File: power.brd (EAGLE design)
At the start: 120 x 120 mm, 34 parts, among them CN1 21700, CN2 21700, CN5 15PIN 0.5MM, Q1 IRLML6244, Q2 IRLML6244, U1 MAX17320G20+

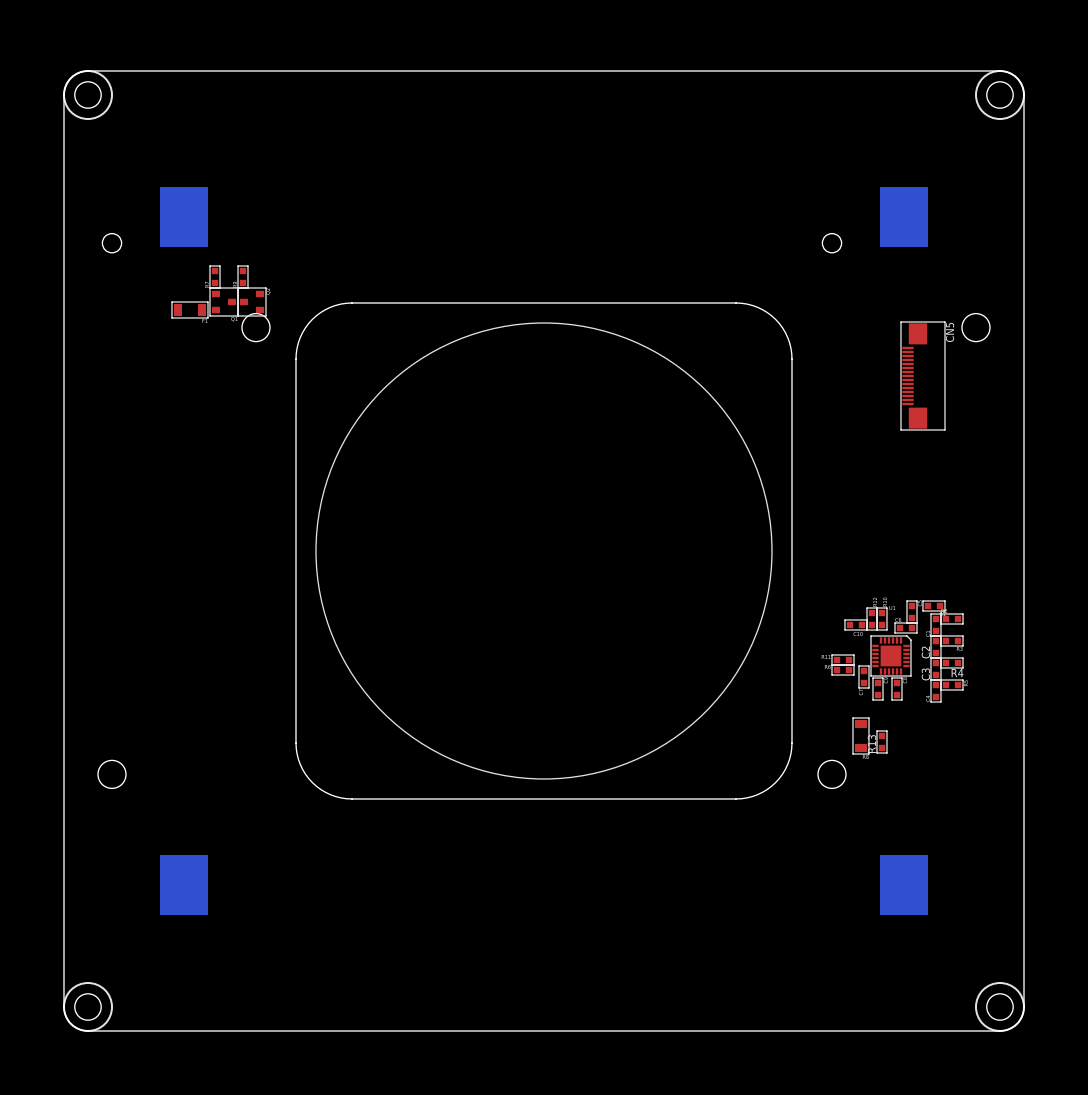
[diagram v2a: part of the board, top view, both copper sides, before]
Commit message: Progress
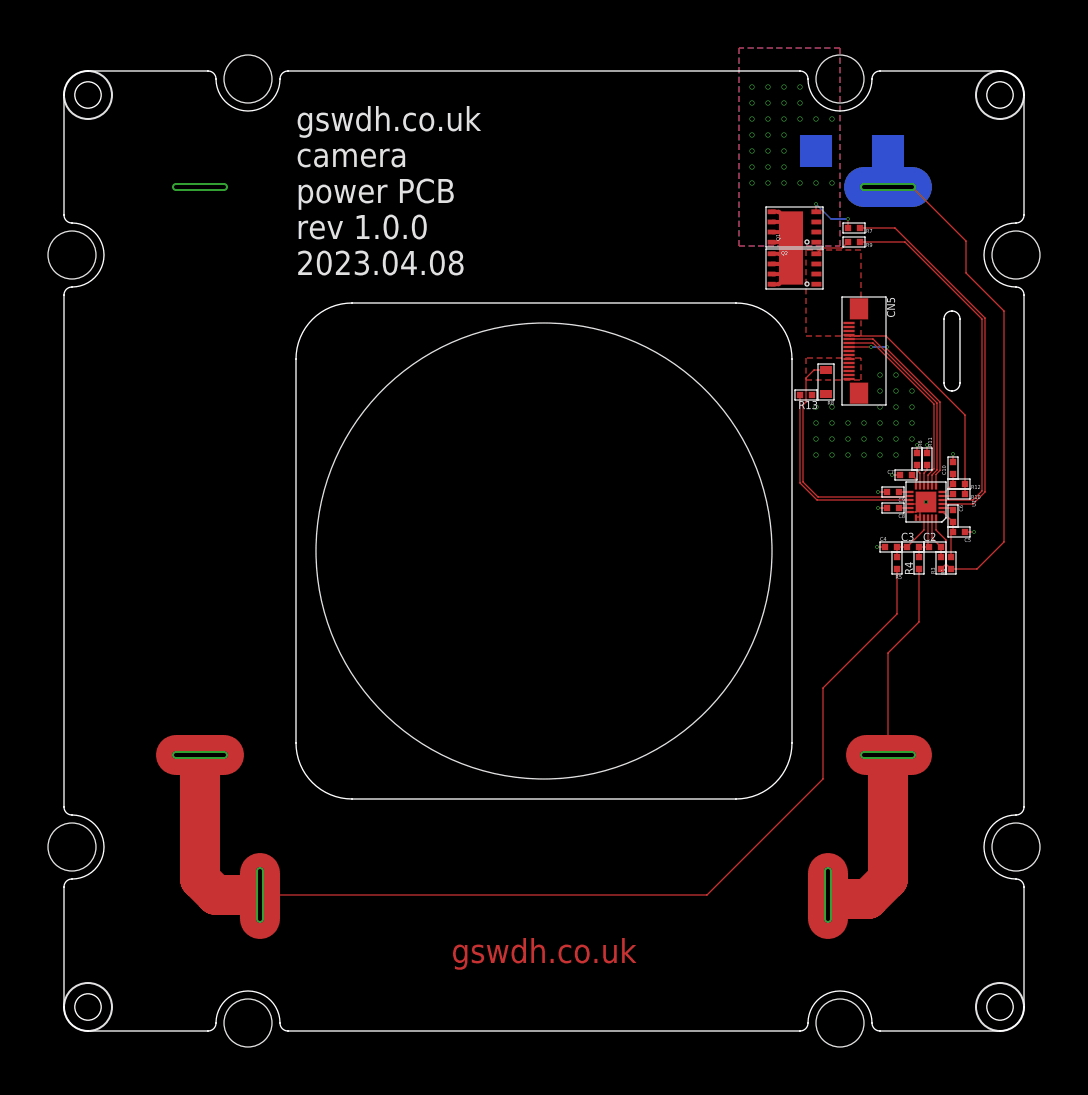
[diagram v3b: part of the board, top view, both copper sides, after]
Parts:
- removed C1: 100nF 16V, CAPACITORS:0603
- removed R2: 47R, r_0603:0603
- added CN3: 21700, CONNECTORs:21700_TABBED
- CN1, CN2: device CONNECTORs:1122 -> CONNECTORs:21700_TABBED
- F1: value 1A Fast -> 20A; device FUSES:1206 -> FUSES:0678H
- Q1, Q2: value IRLML6244 -> SIRA36DP-T1-GE3; device TRANSISTORs:SOT23-3 -> TRANSISTORs:SO8_POWERPAK
- moved F1 85.1 mm to (38.5, 50.0), flipped to the bottom, turned to 0 degrees
- moved R7 80.1 mm to (38.8, 40.4), turned to 180 degrees
- moved R9 76.5 mm to (38.8, 38.6), turned to 180 degrees
- moved Q1 72.0 mm to (31.4, 40.5), turned to 180 degrees
- moved Q2 68.0 mm to (31.4, 35.2), turned to 180 degrees
- moved CN2 62.2 mm to (0.00, -43.0)
- moved R8 44.5 mm to (35.2, 21.1)
- moved R13 44.4 mm to (32.8, 19.5), turned to 180 degrees
- moved R6 28.0 mm to (46.6, 11.5), turned to 270 degrees
- moved R11 27.2 mm to (47.9, 11.5), turned to 270 degrees
- moved C7 25.8 mm to (45.2, 9.50), turned to 180 degrees
- moved C9 24.7 mm to (43.6, 7.38), turned to 180 degrees
- moved C10 23.1 mm to (51.1, 10.4), turned to 270 degrees
- moved C8 22.6 mm to (43.6, 5.38), turned to 180 degrees
- moved R12 20.1 mm to (51.9, 8.38), turned to 0 degrees
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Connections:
- removed net N$36: F1.1, R1.1, R2.1
- removed net N$4: R3.1
- net N$2: no longer C1.1
- net N$39: now also CN3.P1, CN3.P10, CN3.P11, CN3.P12, CN3.P13, CN3.P14, CN3.P15, CN3.P16, CN3.P17, CN3.P18, CN3.P19, CN3.P2, CN3.P20, CN3.P21, CN3.P22, CN3.P23, CN3.P24, CN3.P25, CN3.P3, CN3.P4, CN3.P5, CN3.P6, CN3.P7, CN3.P8, CN3.P9, F1.1, R1.1, R3.1; no longer C1.2, R2.2
- net N$42: now also Q1.1, Q1.2
- net N$43: now also Q2.4; no longer Q2.1
- net N$5: now also CN2.P1, CN2.P10, CN2.P11, CN2.P12, CN2.P13, CN2.P14, CN2.P15, CN2.P16, CN2.P17, CN2.P18, CN2.P19, CN2.P2, CN2.P20, CN2.P21, CN2.P22, CN2.P23, CN2.P24, CN2.P25, CN2.P3, CN2.P4, CN2.P5, CN2.P6, CN2.P7, CN2.P8, CN2.P9, CN3.N, CN3.N1, CN3.N10, CN3.N11, CN3.N12, CN3.N13, CN3.N14, CN3.N15, CN3.N16, CN3.N17, CN3.N18, CN3.N19, CN3.N2, CN3.N20, CN3.N21, CN3.N22, CN3.N23, CN3.N24, CN3.N3, CN3.N4, CN3.N5, CN3.N6, CN3.N7, CN3.N8, CN3.N9; no longer CN2.+
- net N$57: now also Q1.5, Q1.6, Q1.7, Q1.8, Q1.PAD, Q2.5, Q2.6, Q2.7, Q2.8, Q2.PAD; no longer Q1.2, Q2.2
- net N$58: now also Q1.4; no longer Q1.1
- net PACK_MID: now also CN1.P1, CN1.P10, CN1.P11, CN1.P12, CN1.P13, CN1.P14, CN1.P15, CN1.P16, CN1.P17, CN1.P18, CN1.P19, CN1.P2, CN1.P20, CN1.P21, CN1.P22, CN1.P23, CN1.P24, CN1.P25, CN1.P3, CN1.P4, CN1.P5, CN1.P6, CN1.P7, CN1.P8, CN1.P9, CN2.N, CN2.N1, CN2.N10, CN2.N11, CN2.N12, CN2.N13, CN2.N14, CN2.N15, CN2.N16, CN2.N17, CN2.N18, CN2.N19, CN2.N2, CN2.N20, CN2.N21, CN2.N22, CN2.N23, CN2.N24, CN2.N3, CN2.N4, CN2.N5, CN2.N6, CN2.N7, CN2.N8, CN2.N9; no longer CN1.+, CN2.-
- net PGND: now also CN1.N, CN1.N1, CN1.N10, CN1.N11, CN1.N12, CN1.N13, CN1.N14, CN1.N15, CN1.N16, CN1.N17, CN1.N18, CN1.N19, CN1.N2, CN1.N20, CN1.N21, CN1.N22, CN1.N23, CN1.N24, CN1.N3, CN1.N4, CN1.N5, CN1.N6, CN1.N7, CN1.N8, CN1.N9; no longer CN1.-
- net PWR_VPACK: now also Q2.1, Q2.2
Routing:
- net PACK_MID: track 0.00 -> 142.0 mm
- net N$39: track 0.00 -> 75.7 mm
- net N$5: track 0.00 -> 60.4 mm
- net N$59: track 0.00 -> 48.1 mm
- net N$56: track 0.00 -> 46.2 mm
- net N$57: track 0.00 -> 32.0 mm
- net GND: track 0.00 -> 30.3 mm
- net PWR_VPACK: track 0.00 -> 28.5 mm
- net N$6: track 0.00 -> 25.7 mm
- net BMS_NALERT: track 0.00 -> 25.1 mm, vias 0 -> 2
- net BMS_I2C_SCL: track 0.00 -> 25.0 mm
- net BMS_I2C_SDA: track 0.00 -> 24.4 mm
- net PGND: track 0.00 -> 14.3 mm, vias 0 -> 39
- net N$1: track 0.00 -> 7.05 mm
- net N$58: track 0.00 -> 6.89 mm, vias 0 -> 2
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- added copper zone on layer 1, net GND
- added copper zone on layer 1, net N$42
- added copper zone on layer 16, net N$42
- added copper zone on layer 1, net PWR_VPACK
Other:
- outline, holes or cut-outs redrawn
- board text added: "gswdh.co.uk"
- board text added: "gswdh.co.uk camera power PCB rev 1.0.0 2023.04.08"
